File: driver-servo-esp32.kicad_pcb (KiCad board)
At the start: 2 copper layers, 53.6 x 55.7 mm, 64 parts, among them J1 USB_B, J3 Jack-DC, J5 USB_B, Q1 Q_NPN_BEC, Q2 Q_NPN_BEC, SW1 SW_Push, SW2 SW_Push, SW3 SW_DIP_x01, SW4 SW_DIP_x01, U1 ESP32-PICO-D4, U2 CP2102N-SHORT, U3 AMS1117-3.3, U4 CP2102N-SHORT, U5 74HC245

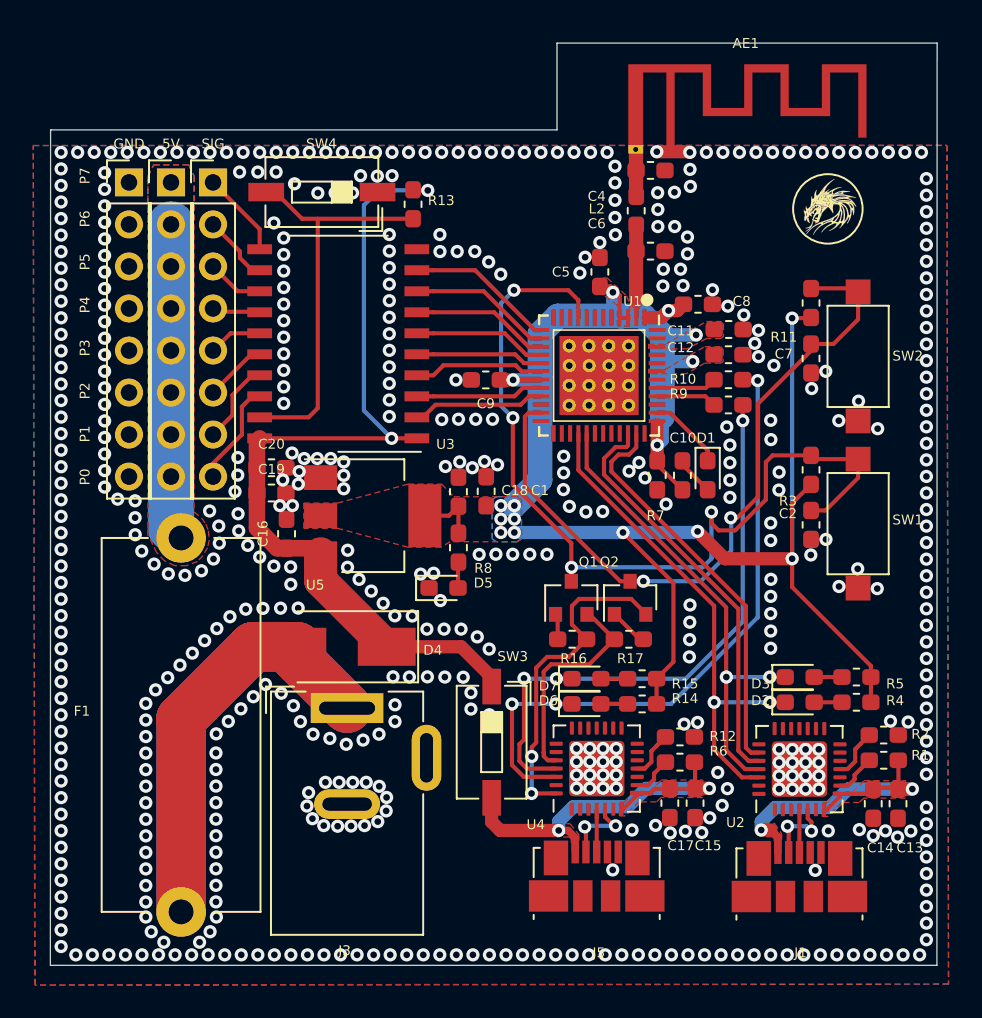
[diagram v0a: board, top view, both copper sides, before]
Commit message: export gerber
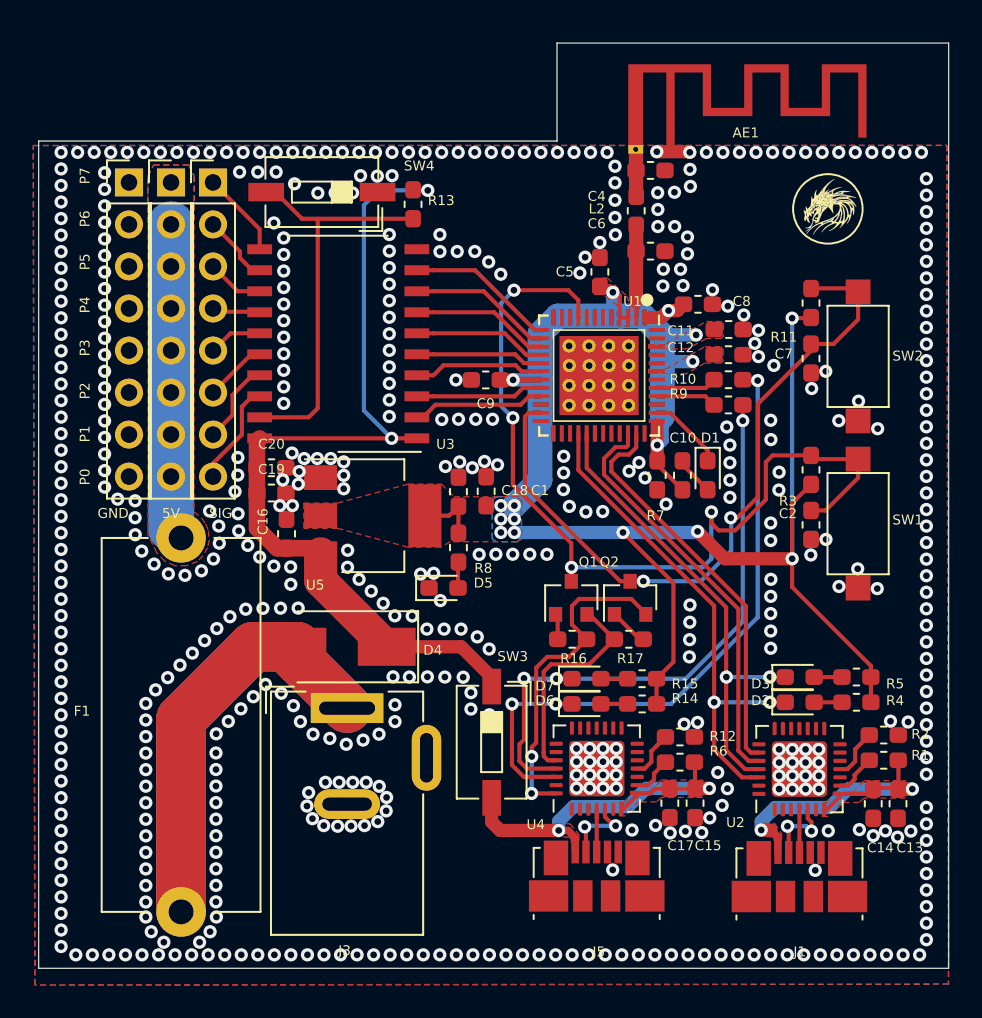
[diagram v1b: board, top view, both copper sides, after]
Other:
- board size 53.6 x 55.7 mm -> 55 x 55.9 mm
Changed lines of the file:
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@@
     (35 F.Paste user hide)
     (36 B.SilkS user hide)
-    (37 F.SilkS user hide)
+    (37 F.SilkS user)
     (38 B.Mask user hide)
     (39 F.Mask user hide)
@@
     (45 Margin user hide)
     (46 B.CrtYd user hide)
-    (47 F.CrtYd user hide)
+    (47 F.CrtYd user)
     (48 B.Fab user hide)
     (49 F.Fab user hide)
@@
       (outputformat 1)
       (mirror false)
-      (drillshape 1)
+      (drillshape 0)
       (scaleselection 1)
-      (outputdirectory ""))
+      (outputdirectory "asset/"))
   )
   (net 0 "")
@@
     (descr "Through hole straight pin header, 1x08, 2.54mm pitch, single row")
     (tags "Through hole pin header THT 1x08 2.54mm single row")
-    (fp_text reference 5V (at 0 -2.33) (layer F.SilkS)
+    (fp_text reference 5V (at 0 20) (layer F.SilkS)
       (effects (font (size 0.6 0.6) (thickness 0.15)))
     )
@@
     (tags "PCB antenna")
     (attr virtual)
-    (fp_text reference AE1 (at 4.55 -6.41) (layer F.SilkS)
+    (fp_text reference AE1 (at 4.55 -1.0059) (layer F.SilkS)
       (effects (font (size 0.6 0.6) (thickness 0.15)))
     )
@@
     (tags "capacitor handsolder")
     (attr smd)
-    (fp_text reference C5 (at 0 -2.3495 180) (layer F.SilkS)
+    (fp_text reference C5 (at 0.01 -2.1205 180) (layer F.SilkS)
       (effects (font (size 0.6 0.6) (thickness 0.15)))
     )
@@
     (tags "capacitor handsolder")
     (attr smd)
-    (fp_text reference C16 (at 0 -1.43 90) (layer F.SilkS)
+    (fp_text reference C16 (at 0.7342 -1.43 90) (layer F.SilkS)
       (effects (font (size 0.6 0.6) (thickness 0.15)))
     )
@@
     (tags "LED handsolder")
     (attr smd)
-    (fp_text reference D1 (at -2.255601 0.100799 180) (layer F.SilkS)
+    (fp_text reference D1 (at -2.255601 -0.165201 180) (layer F.SilkS)
       (effects (font (size 0.6 0.6) (thickness 0.15)))
     )
@@
     (tags "LED handsolder")
     (attr smd)
-    (fp_text reference D6 (at -2.2987 -0.2032) (layer F.SilkS)
+    (fp_text reference D6 (at -2.5077 -0.2032) (layer F.SilkS)
       (effects (font (size 0.6 0.6) (thickness 0.15)))
     )
@@
     (tags "LED handsolder")
     (attr smd)
-    (fp_text reference D7 (at -2.2987 0.4318) (layer F.SilkS)
+    (fp_text reference D7 (at -2.5077 0.4318) (layer F.SilkS)
       (effects (font (size 0.6 0.6) (thickness 0.15)))
     )
@@
     (tags "Micro B USB SMD")
     (attr smd)
-    (fp_text reference J1 (at 0.0658 4.5982 180) (layer F.SilkS)
+    (fp_text reference J1 (at 0.0168 4.5402 180) (layer F.SilkS)
       (effects (font (size 0.6 0.6) (thickness 0.15)))
     )
@@
     (descr "Through hole straight pin header, 1x08, 2.54mm pitch, single row")
     (tags "Through hole pin header THT 1x08 2.54mm single row")
-    (fp_text reference GND (at 0 -2.33) (layer F.SilkS)
+    (fp_text reference GND (at -0.96 20) (layer F.SilkS)
       (effects (font (size 0.6 0.6) (thickness 0.15)))
     )
@@
     (tags "Micro B USB SMD")
     (attr smd)
-    (fp_text reference J5 (at 0.1272 4.6296 180) (layer F.SilkS)
+    (fp_text reference J5 (at 0.1272 4.5716 180) (layer F.SilkS)
       (effects (font (size 0.6 0.6) (thickness 0.15)))
     )
@@
     (descr "Through hole straight pin header, 1x08, 2.54mm pitch, single row")
     (tags "Through hole pin header THT 1x08 2.54mm single row")
-    (fp_text reference SIG (at 0 -2.33) (layer F.SilkS)
+    (fp_text reference SIG (at 0.46 20) (layer F.SilkS)
       (effects (font (size 0.6 0.6) (thickness 0.15)))
     )
@@
     (tags "SMD DIP Switch SPST Slide 6.73mm 264mil SMD LowProfile JPin")
     (attr smd)
-    (fp_text reference SW4 (at 0.0254 2.921) (layer F.SilkS)
+    (fp_text reference SW4 (at -5.8816 1.584) (layer F.SilkS)
       (effects (font (size 0.6 0.6) (thickness 0.15)))
     )
@@
     (effects (font (size 0.6 0.6) (thickness 0.15)))
   )
-  (gr_line (start 123.3297 91.5797) (end 146.304 91.5797) (layer Edge.Cuts) (width 0.05))
-  (gr_line (start 123.3297 96.825) (end 123.3297 91.5797) (layer Edge.Cuts) (width 0.05))
-  (gr_line (start 92.7227 96.825) (end 123.3297 96.825) (layer Edge.Cuts) (width 0.05))
-  (gr_line (start 92.71 147.32) (end 92.7227 96.825) (layer Edge.Cuts) (width 0.05))
-  (gr_line (start 146.2913 147.32) (end 92.71 147.32) (layer Edge.Cuts) (width 0.05))
-  (gr_line (start 146.304 91.5797) (end 146.2913 147.32) (layer Edge.Cuts) (width 0.05))
+  (gr_line (start 123.3297 91.5797) (end 147 91.5797) (layer Edge.Cuts) (width 0.05))
+  (gr_line (start 123.3297 97.5) (end 123.3297 91.5797) (layer Edge.Cuts) (width 0.05))
+  (gr_line (start 92 97.5) (end 123.3297 97.5) (layer Edge.Cuts) (width 0.05))
+  (gr_line (start 91.9988 147.5) (end 92 97.5) (layer Edge.Cuts) (width 0.05))
+  (gr_line (start 147 147.5) (end 92 147.5) (layer Edge.Cuts) (width 0.05))
+  (gr_line (start 147 91.5797) (end 147 147.5) (layer Edge.Cuts) (width 0.05))
   (via (at 131.0132 132.7404) (size 0.8) (drill 0.4) (layers F.Cu B.Cu) (net 1))
   (via (at 131.826 132.6388) (size 0.8) (drill 0.4) (layers F.Cu B.Cu) (net 1))
